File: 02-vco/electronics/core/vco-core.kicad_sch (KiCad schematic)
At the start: 7 parts, among them J1 Conn_01x04, J2 Conn_02x05_Odd_Even, J6 Conn_02x02_Counter_Clockwise

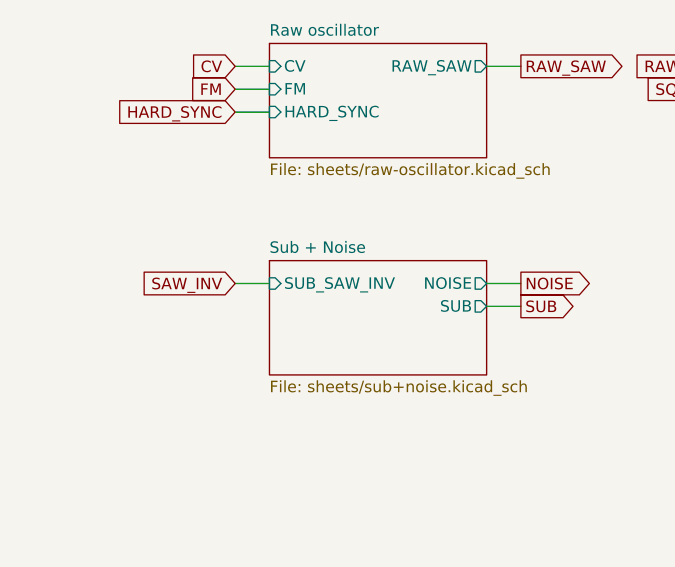
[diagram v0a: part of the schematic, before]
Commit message: Updated sub circuit
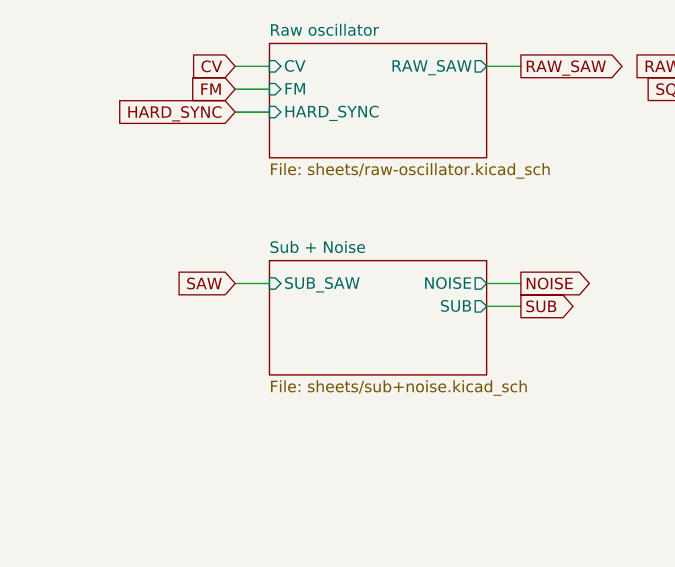
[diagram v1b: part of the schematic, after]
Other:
- sheet Sub + Noise ports: added SUB_SAW; removed SUB_SAW_INV
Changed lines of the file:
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@@
 		)
 	)
-	(global_label "SAW_INV"
+	(global_label "SAW"
 		(shape input)
 		(at 38.1 101.6 180)
@@
 		)
 		(property "Intersheetrefs" "${INTERSHEET_REFS}"
-			(at 27.3738 101.6 0)
+			(at 31.3653 101.6 0)
 			(effects
 				(font
@@
 			)
 		)
-		(pin "SUB_SAW_INV" input
+		(pin "SUB_SAW" input
 			(at 41.91 101.6 180)
 			(effects
